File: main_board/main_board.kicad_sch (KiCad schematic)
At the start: 55 parts, among them J1 USB4105-GF-A-060, Q3 NX3008PBK,215, U1 SSD1306, U2 ESP32-S2-SOLO, U3 TLV62568PDRLT, U4 MCP73832, U5 DW01, U6 8205A, U7 MAX17055, Y1 SC32S-7PF20PPM

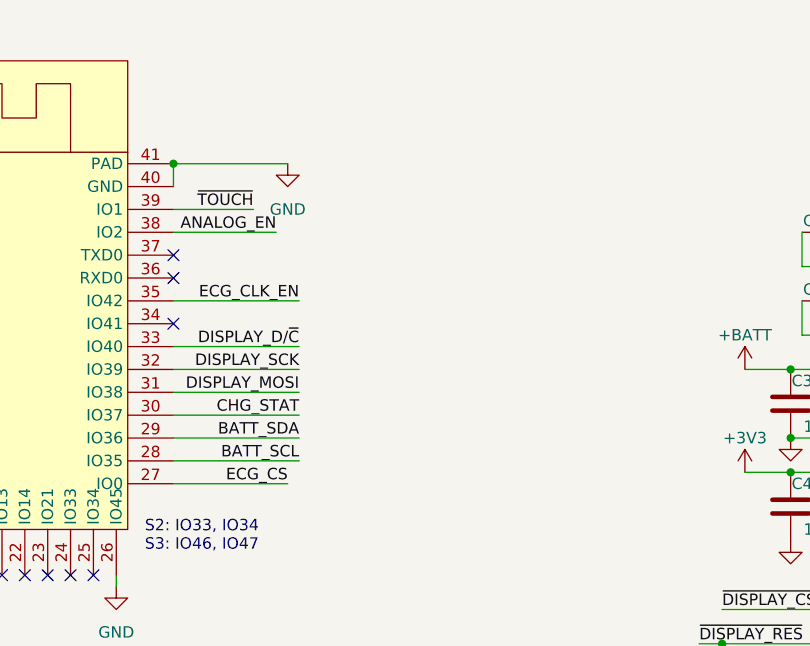
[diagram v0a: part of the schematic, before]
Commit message: Clean up
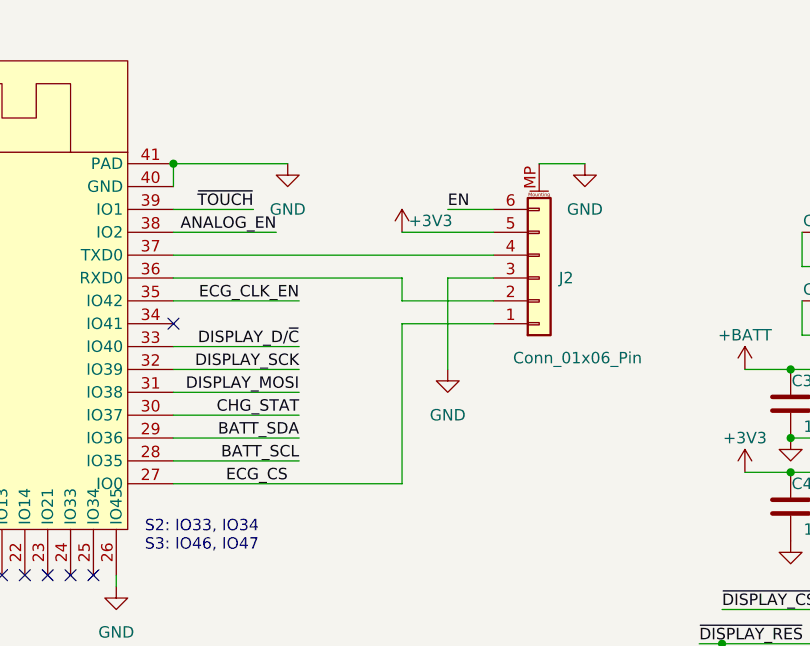
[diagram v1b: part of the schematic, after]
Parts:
- added J2: Conn_01x06_Pin, Connector_Molex:Molex_Pico-Clasp_501331-0607_1x06-1MP_P1.00mm_Vertical, symbol Connector_Generic_MountingPin:Conn_01x06_MountingPin
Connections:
- net +3V3: now also J2.5 (Pin_5)
- net ECG_CS: now also J2.1 (Pin_1)
- net EN: now also J2.6 (Pin_6)
- net GND: now also J2.3 (Pin_3), J2.MP (MountPin)
- net at U2.36 (RXD0): now also J2.2 (Pin_2)
- net at U2.37 (TXD0): now also J2.4 (Pin_4)
- no-connect marks 19 -> 17
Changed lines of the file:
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@@
   (no_connect (at 138.43 78.74))
   (no_connect (at 153.67 78.74))
-  (no_connect (at 170.18 45.72))
   (no_connect (at 198.12 144.78))
   (no_connect (at 148.59 78.74))
-  (no_connect (at 170.18 43.18))
   (no_connect (at 139.7 170.18))
   (no_connect (at 143.51 78.74))
@@
     (stroke (width 0) (type default))
   )
+  (wire (pts (xy 195.58 50.8) (xy 205.74 50.8))
+    (stroke (width 0) (type default))
+  )
   (wire (pts (xy 200.66 134.62) (xy 200.66 135.89))
     (stroke (width 0) (type default))
@@
     (stroke (width 0) (type default))
   )
+  (wire (pts (xy 195.58 68.58) (xy 195.58 50.8))
+    (stroke (width 0) (type default))
+  )
   (wire (pts (xy 74.93 120.65) (xy 74.93 121.92))
     (stroke (width 0) (type default))
@@
     (stroke (width 0) (type default))
   )
+  (wire (pts (xy 200.66 45.72) (xy 200.66 55.88))
+    (stroke (width 0) (type default))
+  )
   (wire (pts (xy 198.12 121.92) (xy 201.93 121.92))
     (stroke (width 0) (type default))
@@
     (stroke (width 0) (type default))
   )
+  (wire (pts (xy 200.66 38.1) (xy 205.74 38.1))
+    (stroke (width 0) (type default))
+  )
   (wire (pts (xy 137.16 177.8) (xy 137.16 180.34))
     (stroke (width 0) (type default))
@@
     (stroke (width 0) (type default))
   )
+  (wire (pts (xy 210.82 33.02) (xy 215.9 33.02))
+    (stroke (width 0) (type default))
+  )
   (wire (pts (xy 238.76 90.17) (xy 254 90.17))
     (stroke (width 0) (type default))
@@
     (stroke (width 0) (type default))
   )
+  (wire (pts (xy 195.58 40.64) (xy 205.74 40.64))
+    (stroke (width 0) (type default))
+  )
   (wire (pts (xy 254 71.12) (xy 246.38 71.12))
     (stroke (width 0) (type default))
@@
     (stroke (width 0) (type default))
   )
+  (wire (pts (xy 170.18 45.72) (xy 195.58 45.72))
+    (stroke (width 0) (type default))
+  )
   (wire (pts (xy 73.66 165.1) (xy 74.93 165.1))
     (stroke (width 0) (type default))
@@
     (stroke (width 0) (type default))
   )
+  (wire (pts (xy 195.58 48.26) (xy 205.74 48.26))
+    (stroke (width 0) (type default))
+  )
   (wire (pts (xy 139.7 175.26) (xy 129.54 175.26))
     (stroke (width 0) (type default))
@@
     (stroke (width 0) (type default))
   )
+  (wire (pts (xy 170.18 43.18) (xy 205.74 43.18))
+    (stroke (width 0) (type default))
+  )
   (wire (pts (xy 247.65 48.26) (xy 254 48.26))
     (stroke (width 0) (type default))
@@
     (stroke (width 0) (type default))
   )
+  (wire (pts (xy 195.58 45.72) (xy 195.58 48.26))
+    (stroke (width 0) (type default))
+  )
   (wire (pts (xy 120.65 138.43) (xy 120.65 139.7))
     (stroke (width 0) (type default))
@@
     (stroke (width 0) (type default))
   )
-  (wire (pts (xy 170.18 68.58) (xy 182.88 68.58))
+  (wire (pts (xy 170.18 68.58) (xy 195.58 68.58))
     (stroke (width 0) (type default))
   )
@@
   )
   (wire (pts (xy 69.85 45.72) (xy 129.54 45.72))
+    (stroke (width 0) (type default))
+  )
+  (wire (pts (xy 205.74 45.72) (xy 200.66 45.72))
     (stroke (width 0) (type default))
   )
@@
   (label "BATT_SCL" (at 165.1 172.72 180) (fields_autoplaced)
     (effects (font (size 1.27 1.27)) (justify right bottom))
+  )
+  (label "EN" (at 200.66 38.1 0) (fields_autoplaced)
+    (effects (font (size 1.27 1.27)) (justify left bottom))
   )
   (label "BATT_SDA" (at 25.4 194.31 0) (fields_autoplaced)
@@
     )
   )
+  (symbol (lib_id "power:GND") (at 200.66 55.88 0) (mirror y) (unit 1)
+    (in_bom yes) (on_board yes) (dnp no)
+    (property "Reference" "#PWR012" (at 200.66 62.23 0)
+      (effects (font (size 1.27 1.27)) hide)
+    )
+    (property "Value" "GND" (at 200.66 60.96 0)
+      (effects (font (size 1.27 1.27)))
+    )
+    (property "Footprint" "" (at 200.66 55.88 0)
+      (effects (font (size 1.27 1.27)) hide)
+    )
+    (property "Datasheet" "" (at 200.66 55.88 0)
+      (effects (font (size 1.27 1.27)) hide)
+    )
+    (pin "1")
+    (instances
+      (project "main_board"
+        (path "/e55848cd-275a-4b5e-8e68-b5d8d07c8d31"
+          (reference "#PWR012") (unit 1)
+        )
+      )
+    )
+  )
   (symbol (lib_id "Device:R") (at 148.59 186.69 270) (unit 1)
     (in_bom yes) (on_board yes) (dnp no)
@@
     )
   )
+  (symbol (lib_id "power:GND") (at 215.9 33.02 0) (mirror y) (unit 1)
+    (in_bom yes) (on_board yes) (dnp no)
+    (property "Reference" "#PWR013" (at 215.9 39.37 0)
+      (effects (font (size 1.27 1.27)) hide)
+    )
+    (property "Value" "GND" (at 215.9 38.1 0)
+      (effects (font (size 1.27 1.27)))
+    )
+    (property "Footprint" "" (at 215.9 33.02 0)
+      (effects (font (size 1.27 1.27)) hide)
+    )
+    (property "Datasheet" "" (at 215.9 33.02 0)
+      (effects (font (size 1.27 1.27)) hide)
+    )
+    (pin "1")
+    (instances
+      (project "main_board"
+        (path "/e55848cd-275a-4b5e-8e68-b5d8d07c8d31"
+          (reference "#PWR013") (unit 1)
+        )
+      )
+    )
+  )
   (symbol (lib_id "Device:C") (at 243.84 40.64 90) (unit 1)
     (in_bom yes) (on_board yes) (dnp no)
@@
         (path "/e55848cd-275a-4b5e-8e68-b5d8d07c8d31"
           (reference "C13") (unit 1)
+        )
+      )
+    )
+  )
+  (symbol (lib_id "Connector_Generic_MountingPin:Conn_01x06_MountingPin") (at 210.82 45.72 0) (mirror x) (unit 1)
+    (in_bom yes) (on_board yes) (dnp no)
+    (property "Reference" "J2" (at 214.63 45.72 0)
+      (effects (font (size 1.27 1.27)) (justify right))
+    )
+    (property "Value" "Conn_01x06_Pin" (at 222.25 54.61 0)
+      (effects (font (size 1.27 1.27)) (justify right))
+    )
+    (property "Footprint" "Connector_Molex:Molex_Pico-Clasp_501331-0607_1x06-1MP_P1.00mm_Vertical" (at 210.82 45.72 0)
+      (effects (font (size 1.27 1.27)) hide)
+    )
+    (property "Datasheet" "~" (at 210.82 45.72 0)
+      (effects (font (size 1.27 1.27)) hide)
+    )
+    (pin "1")
+    (pin "2")
+    (pin "3")
+    (pin "4")
+    (pin "5")
+    (pin "6")
+    (pin "MP")
+    (instances
+      (project "main_board"
+        (path "/e55848cd-275a-4b5e-8e68-b5d8d07c8d31"
+          (reference "J2") (unit 1)
         )
       )
@@
         )
       )
+    )
+  )
+  (symbol (lib_id "power:+3V3") (at 195.58 40.64 0) (unit 1)
+    (in_bom yes) (on_board yes) (dnp no)
+    (property "Reference" "#PWR011" (at 195.58 44.45 0)
+      (effects (font (size 1.27 1.27)) hide)
+    )
+    (property "Value" "+3V3" (at 198.755 39.37 0)
+      (effects (font (size 1.27 1.27)))
+    )
+    (property "Footprint" "" (at 195.58 40.64 0)
+      (effects (font (size 1.27 1.27)) hide)
+    )
+    (property "Datasheet" "" (at 195.58 40.64 0)
+      (effects (font (size 1.27 1.27)) hide)
+    )
+    (pin "1")
+    (instances
+      (project "main_board"
+        (path "/e55848cd-275a-4b5e-8e68-b5d8d07c8d31"
+          (reference "#PWR011") (unit 1)
+        )
+      )
